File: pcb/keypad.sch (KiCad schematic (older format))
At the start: 14 parts, among them SW700 SW_Push, SW701 SW_Push, SW702 SW_Push, SW703 SW_Push, SW704 SW_Push, SW705 SW_Push, SW706 SW_Push, SW707 SW_Push, U100 MCIMX7S5EVM08SC

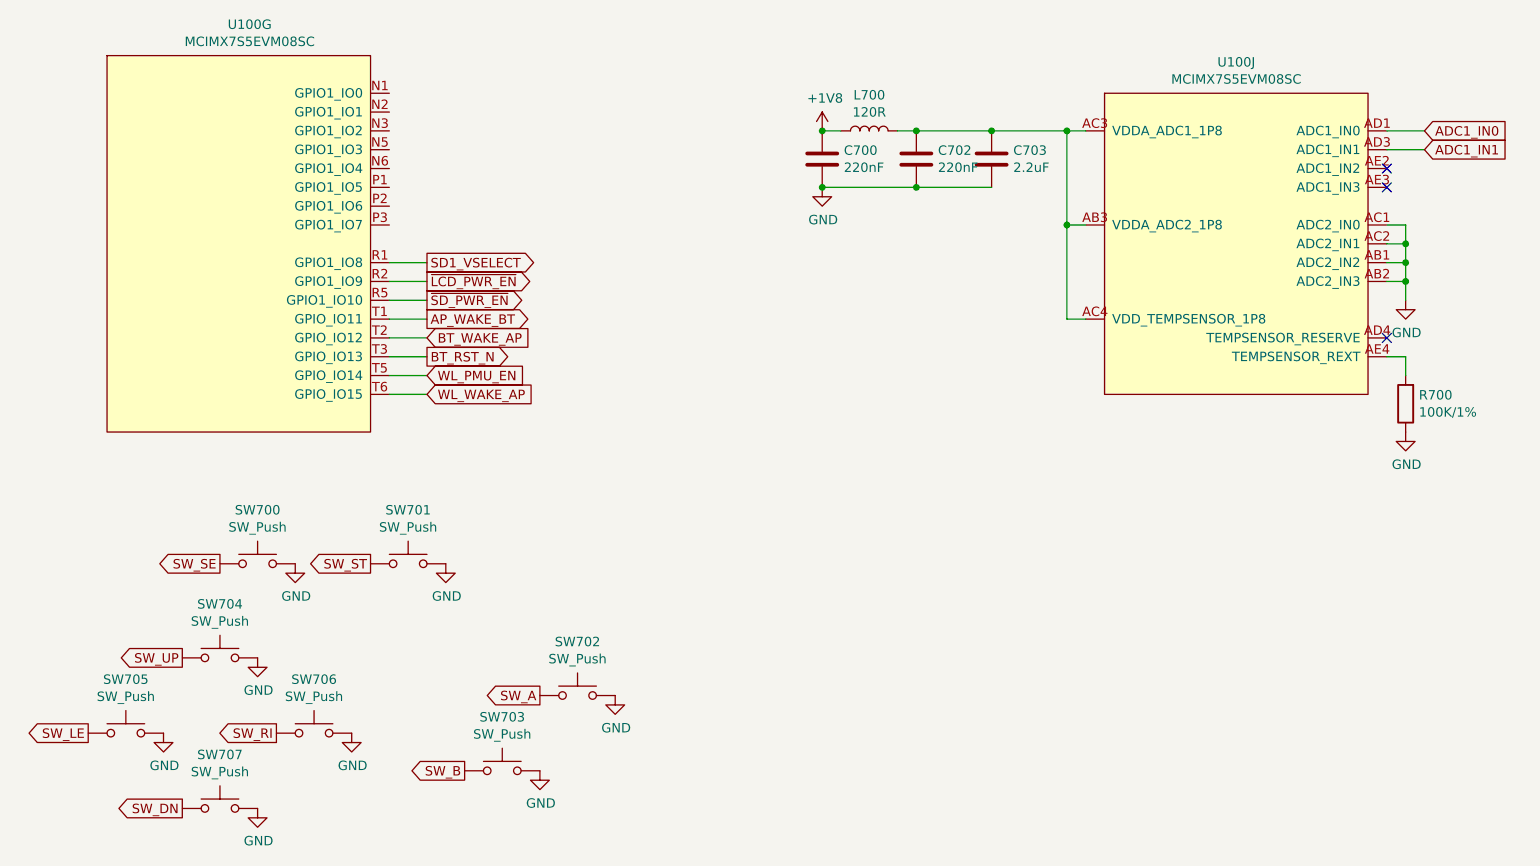
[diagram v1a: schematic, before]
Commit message: pcb: rev 0.1
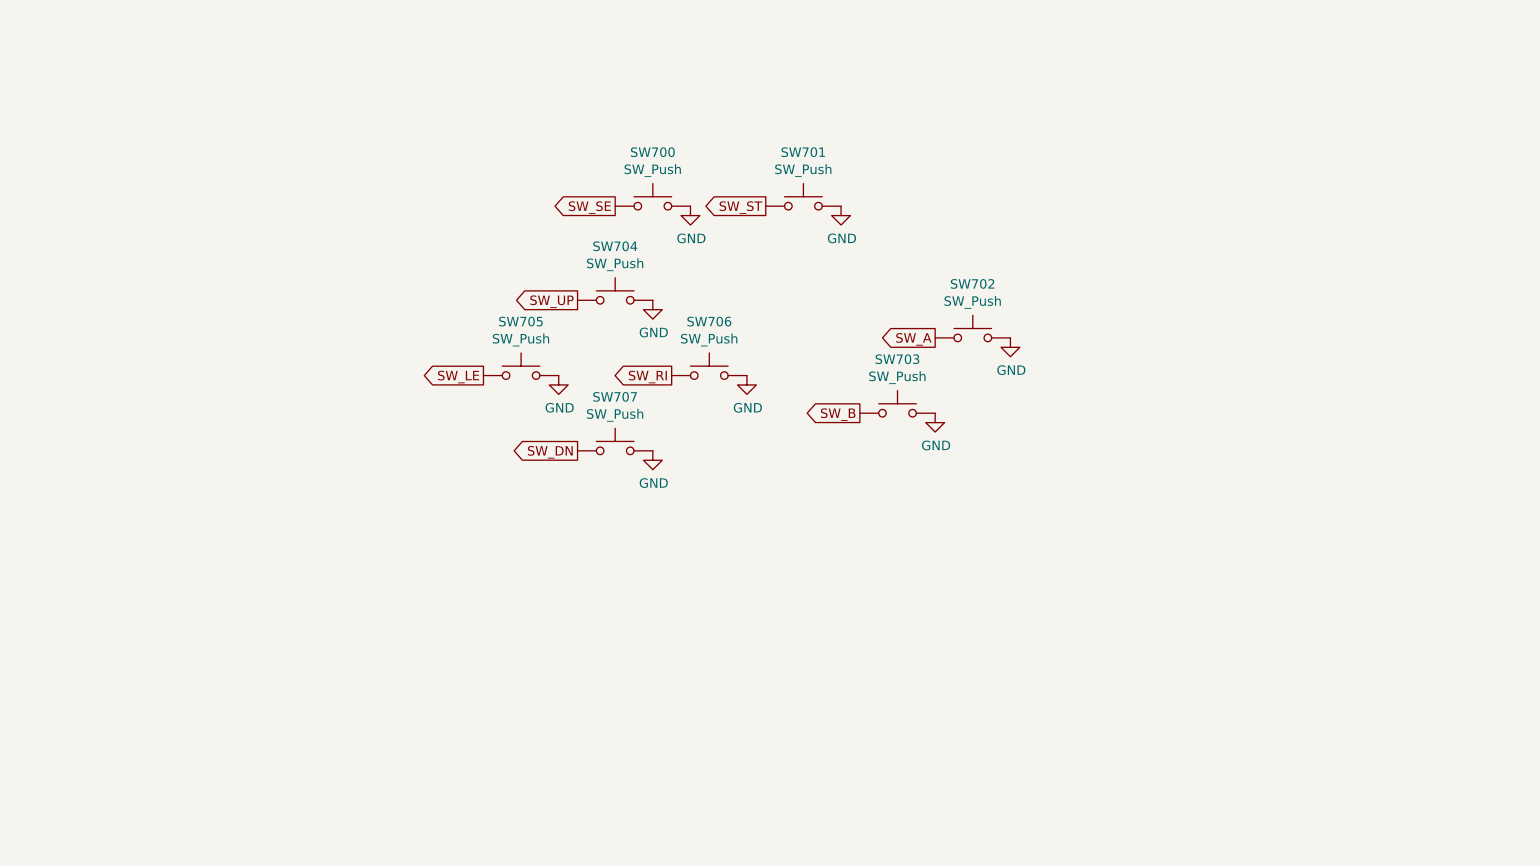
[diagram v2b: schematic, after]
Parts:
- removed C700, C702: 220nF, Capacitor_SMD:C_0402_1005Metric, symbol Device:C
- removed C703: 2.2uF, Capacitor_SMD:C_0402_1005Metric, symbol Device:C
- removed L700: 120R, Inductor_SMD:L_0603_1608Metric, symbol Device:L
- removed R700: 100K/1%, Resistor_SMD:R_0603_1608Metric, symbol Device:R
- removed U100: MCIMX7S5EVM08SC, footprints:BGA-541_25x25_19.0x19.0mm, symbol symbols:MCIMX7S5EVM08SC
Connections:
- no-connect marks 3 -> 0
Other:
- moved on the sheet: SW700, SW701, SW702, SW703, SW704, SW705, SW706, SW707
